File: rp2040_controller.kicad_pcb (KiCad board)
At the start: 4 copper layers, 19 x 29.5 mm, 28 parts, among them J7 rp2040_controller, U1 RP2040, U2 AP2112K-3.3, U3 W25Q64JV, Y1 XYDBPCNANF-12MHZ

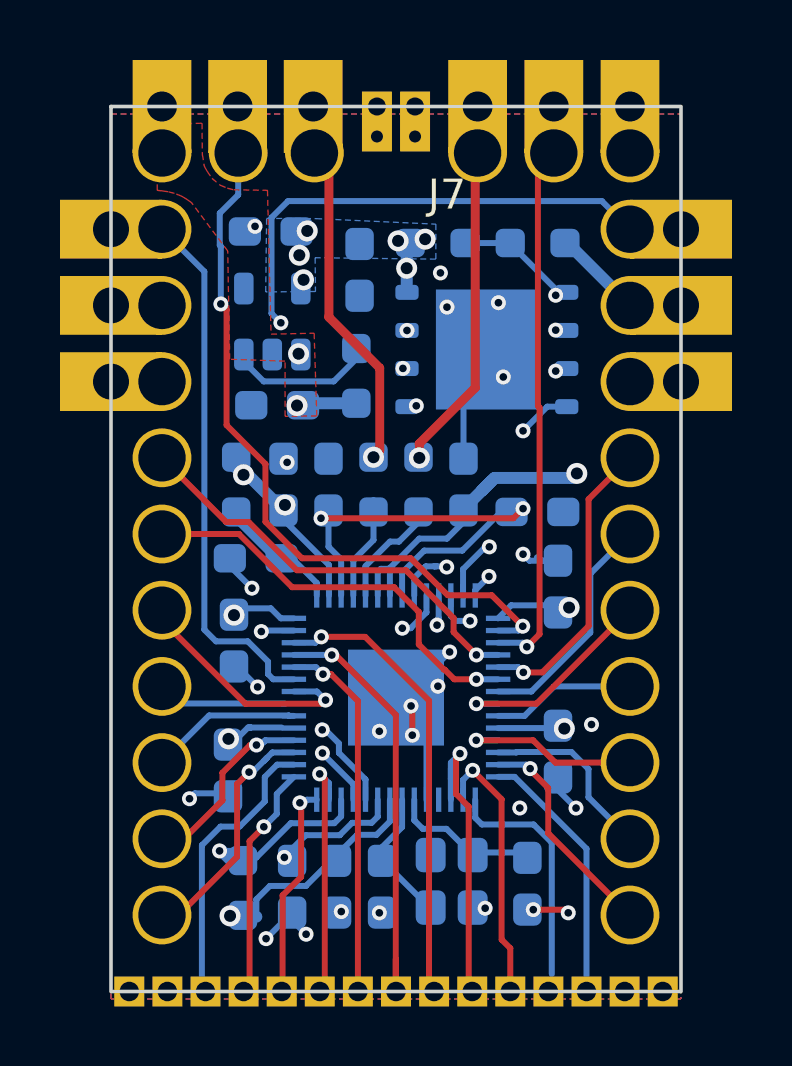
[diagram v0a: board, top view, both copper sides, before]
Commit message: Kicad 7
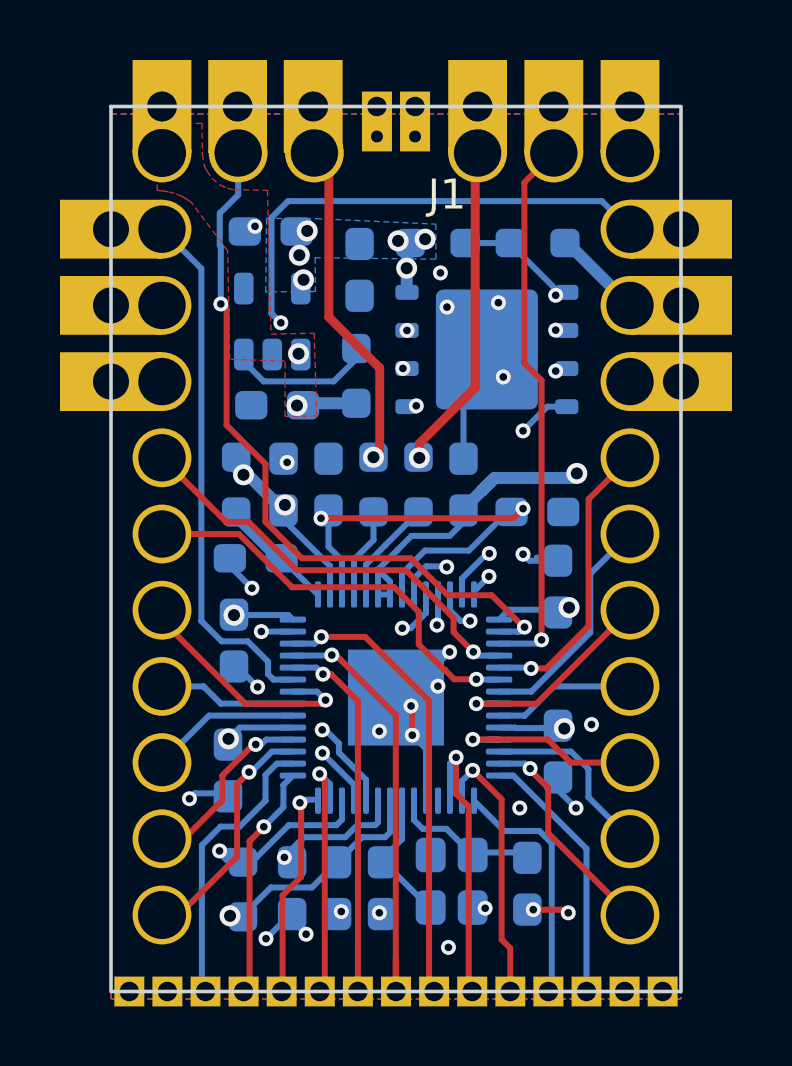
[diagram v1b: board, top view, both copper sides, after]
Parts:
- C1, C10, C11, C12, C13, C14, C15, C16, C2, C3, C4, C5, C6, C7, C8, C9: footprint Capacitor_SMD_AKL:C_0603_1608Metric_Pad1.08x0.95mm -> PCM_Capacitor_SMD_AKL:C_0603_1608Metric_Pad1.08x0.95mm
- R1, R2, R3, R4, R5, R8, R9: footprint Resistor_SMD_AKL:R_0603_1608Metric_Pad0.98x0.95mm_HandSolder -> PCM_Resistor_SMD_AKL:R_0603_1608Metric_Pad0.98x0.95mm_HandSolder
- U1: footprint rp2040:RP2040 -> Package_DFN_QFN:QFN-56-1EP_7x7mm_P0.4mm_EP3.2x3.2mm
- U2: footprint Package_TO_SOT_SMD_AKL:SOT-23-5 -> PCM_Package_TO_SOT_SMD_AKL:SOT-23-5
- U3: footprint Package_SON:WSON-8-1EP_6x5mm_P1.27mm_EP3.4x4mm -> PCM_Package_SON_AKL:WSON-8-1EP_6x5mm_P1.27mm_EP3.4x4mm
- Y1: footprint Crystal_AKL:Crystal_SMD_2520-4Pin_2.5x2.0mm -> PCM_Crystal_AKL:Crystal_SMD_2520-4Pin_2.5x2.0mm
- renumbered J7 to J1
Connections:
- net /USB_N renamed /DM
- net /USB_P renamed /DP
- net /XIN renamed Net-(U1-XIN)
- net /XOUT renamed Net-(U1-XOUT)
- Y1 pad 2: unconnected-(Y1-Pad2) -> GND
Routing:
- net /GPIO1/I2C0_SCL: track 17.2 -> 18.3 mm
- net /GPIO23: track 3.52 -> 4.60 mm
- net +3V3: track 32.9 -> 33.9 mm
- net /DM: track 11.1 -> 10.4 mm
- net /GPIO14: track 9.81 -> 9.14 mm
- net GND: vias 26 -> 27
